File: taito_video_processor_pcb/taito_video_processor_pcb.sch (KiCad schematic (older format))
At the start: 237 parts, among them J1 14pin, J19 2pin, J2 14pin, J3 50pin, J6 50pin, Q1 2N3904, Q2 2N3904, Q3 2N3904, Q4 2N3904, Q5 2N3904, Q6 2N3904, Q7 2N3904, Q8 2N3905, SW1 SW_Push, U1 245_1, U10 4116, U100 LS00, U101 LS08, U102 LS10, U103 LS00, U104 157_1, U105 299_1, U106 299_1, U107 299_1, U108 299_1, U109 299_1, U11 4116, U110 299_1, U12 4116, U13 4116, U14 4116, U15 4116, U16 4116, U17 4116, U18 68A45, U19 86_2, U2 245_1, U20 86_1, U21 157_1, U22 LS32, U23 161_1, U24 LS04, U25 374_1, U26 4116, U27 4116, U28 4116, U29 4116, U3 2114, U30 4116, U31 4116, U32 4116, U33 4116, U34 LS374, U35 153_1, U36 LS74, U37 LS08, U38 74S113, U39 LS04, U4 2114, U40 7417, U41 4116, U42 4116, U43 4116, U44 4116, U45 4116, U46 4116, U47 4116, U48 4116, U49 LS32, U5 157_1, U50 86_3, U51 LS86, U52 153_1, U53 153_1, U54 153_1, U55 157_1, U56 2148_1, U57 2148_2, U58 7417, U59 4116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

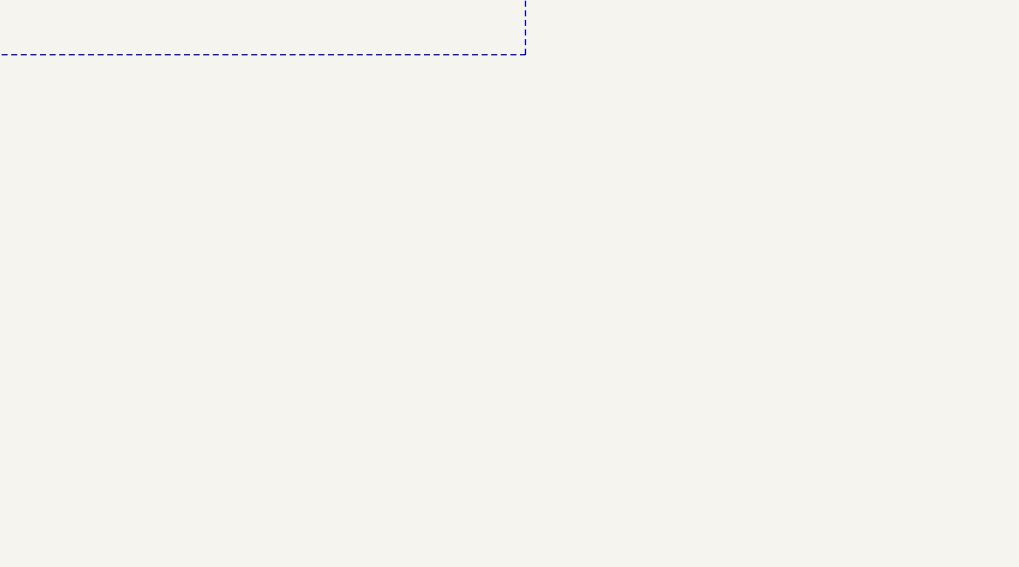
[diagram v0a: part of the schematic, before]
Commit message: Continued layout
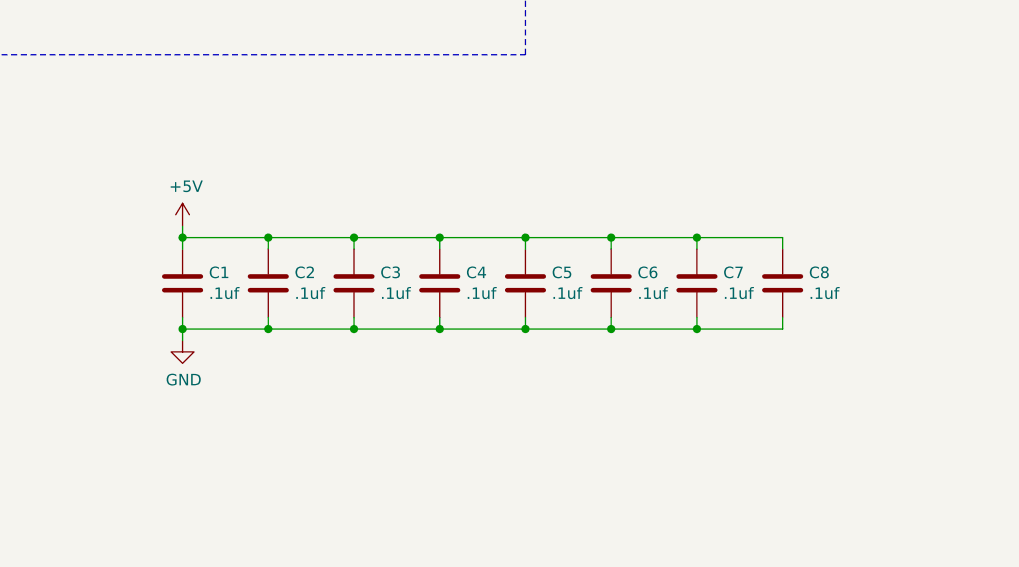
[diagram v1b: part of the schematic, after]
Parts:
- added C1, C2, C3, C4, C5, C6, C7, C8: .1uf, symbol Device:C
- J3, J6: footprint (none) -> taito_video_processor_pcb:50Pin
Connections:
- net +5V: now also C1.1, C2.1, C3.1, C4.1, C5.1, C6.1, C7.1, C8.1
- net GND: now also C1.2, C2.2, C3.2, C4.2, C5.2, C6.2, C7.2, C8.2
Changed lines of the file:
@@
 F 0 "J3" H 1400 3675 30  0000 L CNN
 F 1 "50pin" V 1425 3450 30  0000 L CNN
-F 2 "" H 1425 3425 30  0001 C CNN
+F 2 "taito_video_processor_pcb:50Pin" H 1425 3425 30  0001 C CNN
 F 3 "" H 1425 3425 30  0001 C CNN
 	1    1425 3425
@@
 F 0 "J6" H 31603 13430 30  0000 L CNN
 F 1 "50pin" H 31603 13370 30  0000 L CNN
-F 2 "" H 31525 13375 30  0001 C CNN
+F 2 "taito_video_processor_pcb:50Pin" H 31525 13375 30  0001 C CNN
 F 3 "" H 31525 13375 30  0001 C CNN
 	1    31525 13375
@@
 Wire Notes Line
 	28900 16275 28900 10600
+$Comp
+L Device:C C4
+U 1 1 61171227
+P 28525 17275
+F 0 "C4" H 28640 17321 50  0000 L CNN
+F 1 ".1uf" H 28640 17230 50  0000 L CNN
+F 2 "" H 28563 17125 50  0001 C CNN
+F 3 "~" H 28525 17275 50  0001 C CNN
+	1    28525 17275
+	1    0    0    -1
+$EndComp
+$Comp
+L Device:C C5
+U 1 1 61175975
+P 28900 17275
+F 0 "C5" H 29015 17321 50  0000 L CNN
+F 1 ".1uf" H 29015 17230 50  0000 L CNN
+F 2 "" H 28938 17125 50  0001 C CNN
+F 3 "~" H 28900 17275 50  0001 C CNN
+	1    28900 17275
+	1    0    0    -1
+$EndComp
+$Comp
+L Device:C C6
+U 1 1 61179FCE
+P 29275 17275
+F 0 "C6" H 29390 17321 50  0000 L CNN
+F 1 ".1uf" H 29390 17230 50  0000 L CNN
+F 2 "" H 29313 17125 50  0001 C CNN
+F 3 "~" H 29275 17275 50  0001 C CNN
+	1    29275 17275
+	1    0    0    -1
+$EndComp
+$Comp
+L Device:C C7
+U 1 1 6117E636
+P 29650 17275
+F 0 "C7" H 29765 17321 50  0000 L CNN
+F 1 ".1uf" H 29765 17230 50  0000 L CNN
+F 2 "" H 29688 17125 50  0001 C CNN
+F 3 "~" H 29650 17275 50  0001 C CNN
+	1    29650 17275
+	1    0    0    -1
+$EndComp
+$Comp
+L Device:C C8
+U 1 1 61182C28
+P 30025 17275
+F 0 "C8" H 30140 17321 50  0000 L CNN
+F 1 ".1uf" H 30140 17230 50  0000 L CNN
+F 2 "" H 30063 17125 50  0001 C CNN
+F 3 "~" H 30025 17275 50  0001 C CNN
+	1    30025 17275
+	1    0    0    -1
+$EndComp
+$Comp
+L Device:C C3
+U 1 1 6116CBF6
+P 28150 17275
+F 0 "C3" H 28265 17321 50  0000 L CNN
+F 1 ".1uf" H 28265 17230 50  0000 L CNN
+F 2 "" H 28188 17125 50  0001 C CNN
+F 3 "~" H 28150 17275 50  0001 C CNN
+	1    28150 17275
+	1    0    0    -1
+$EndComp
+$Comp
+L Device:C C2
+U 1 1 611685A7
+P 27775 17275
+F 0 "C2" H 27890 17321 50  0000 L CNN
+F 1 ".1uf" H 27890 17230 50  0000 L CNN
+F 2 "" H 27813 17125 50  0001 C CNN
+F 3 "~" H 27775 17275 50  0001 C CNN
+	1    27775 17275
+	1    0    0    -1
+$EndComp
+$Comp
+L Device:C C1
+U 1 1 61164136
+P 27400 17275
+F 0 "C1" H 27515 17321 50  0000 L CNN
+F 1 ".1uf" H 27515 17230 50  0000 L CNN
+F 2 "" H 27438 17125 50  0001 C CNN
+F 3 "~" H 27400 17275 50  0001 C CNN
+	1    27400 17275
+	1    0    0    -1
+$EndComp
+$Comp
+L power:+5V #PWR0350
+U 1 1 6152E23F
+P 27400 17025
+F 0 "#PWR0350" H 27400 16875 50  0001 C CNN
+F 1 "+5V" H 27415 17198 50  0000 C CNN
+F 2 "" H 27400 17025 50  0001 C CNN
+F 3 "" H 27400 17025 50  0001 C CNN
+	1    27400 17025
+	1    0    0    -1
+$EndComp
+Wire Wire Line
+	27400 17125 27400 17075
+Wire Wire Line
+	27400 17075 27775 17075
+Wire Wire Line
+	30025 17075 30025 17125
+Wire Wire Line
+	30025 17425 30025 17475
+Wire Wire Line
+	30025 17475 29650 17475
+Wire Wire Line
+	27400 17475 27400 17425
+Wire Wire Line
+	27775 17425 27775 17475
+Connection ~ 27775 17475
+Wire Wire Line
+	27775 17475 27400 17475
+Wire Wire Line
+	28150 17425 28150 17475
+Connection ~ 28150 17475
+Wire Wire Line
+	28150 17475 27775 17475
+Wire Wire Line
+	27775 17125 27775 17075
+Connection ~ 27775 17075
+Wire Wire Line
+	27775 17075 28150 17075
+Wire Wire Line
+	28150 17125 28150 17075
+Connection ~ 28150 17075
+Wire Wire Line
+	28150 17075 28525 17075
+Wire Wire Line
+	28525 17125 28525 17075
+Connection ~ 28525 17075
+Wire Wire Line
+	28525 17075 28900 17075
+Wire Wire Line
+	28900 17125 28900 17075
+Connection ~ 28900 17075
+Wire Wire Line
+	28900 17075 29275 17075
+Wire Wire Line
+	28525 17425 28525 17475
+Connection ~ 28525 17475
+Wire Wire Line
+	28525 17475 28150 17475
+Wire Wire Line
+	28900 17425 28900 17475
+Connection ~ 28900 17475
+Wire Wire Line
+	28900 17475 28525 17475
+Wire Wire Line
+	29650 17125 29650 17075
+Connection ~ 29650 17075
+Wire Wire Line
+	29650 17075 30025 17075
+Wire Wire Line
+	29275 17125 29275 17075
+Connection ~ 29275 17075
+Wire Wire Line
+	29275 17075 29650 17075
+Wire Wire Line
+	29275 17425 29275 17475
+Connection ~ 29275 17475
+Wire Wire Line
+	29275 17475 28900 17475
+Wire Wire Line
+	29650 17425 29650 17475
+Connection ~ 29650 17475
+Wire Wire Line
+	29650 17475 29275 17475
+Wire Wire Line
+	27400 17025 27400 17075
+Connection ~ 27400 17075
+$Comp
+L power:GND #PWR0351
+U 1 1 64BAC149
+P 27400 17525
+F 0 "#PWR0351" H 27400 17275 50  0001 C CNN
+F 1 "GND" H 27405 17352 50  0000 C CNN
+F 2 "" H 27400 17525 50  0001 C CNN
+F 3 "" H 27400 17525 50  0001 C CNN
+	1    27400 17525
+	1    0    0    -1
+$EndComp
+Wire Wire Line
+	27400 17525 27400 17475
+Connection ~ 27400 17475
 $EndSCHEMATC

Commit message: Placed components
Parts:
- added C10, C11, C12, C13, C15, C16, C17, C18, C19, C20, C21, C23, C24, C25, C26, C27, C28, C29, C30, C32, C33, C34, C35, C36, C37, C38, C39, C40, C41, C43, C46, C47, C48, C49, C50, C51, C52, C53, C54, C55, C56, C57, C58, C59, C60, C62, C64, C66, C67, C68, C69, C70, C71, C72, C73, C74, C75, C76, C78, C79, C81, C82, C87: .1uf, taito_video_processor_pcb:GenericComp, symbol Device:C
- added R11, R12, R22, R23, R24, R25, R26, R27, R9: ?, taito_video_processor_pcb:GenericComp, symbol Device:R_US
- C1, C14, C2, C3, C31, C4, C5, C6, C65, C7, C8, R1, R10, R13, R14, R15, R16, R17, R18, R19, R2, R20, R21, R28, R29, R3, R30, R31, R32, R33, R34, R35, R36, R39, R4, R40, R41, R42, R43, R44, R5, R6, R7, R8: footprint (none) -> taito_video_processor_pcb:GenericComp
- C22, C42, C44, C45, C61, C63, C77, C80, C9: footprint (none) -> taito_video_processor_pcb:CapA
- FB1, FB2, FB3, FB4, FB5, FB6, FB7: footprint (none) -> taito_video_processor_pcb:FB
- J1, J2: footprint (none) -> taito_video_processor_pcb:con_14pin
- J19: footprint (none) -> taito_video_processor_pcb:con_2pin
- Q1, Q2, Q3, Q4, Q5, Q6, Q7, Q8: footprint (none) -> taito_video_processor_pcb:Trans
- RP1, RP2, RP3, RP4, RP5: footprint (none) -> taito_video_processor_pcb:RP
- TP1, TP2, TP3, TP4: footprint (none) -> taito_video_processor_pcb:TPA
- Y1: footprint (none) -> taito_video_processor_pcb:Crystal
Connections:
- net +12V: now also C16.1, C18.1, C19.1, C21.1, C36.1, C37.1, C55.1, C59.1, C72.1, C76.1, C87.1
- net +5V: now also C10.1, C11.1, C12.1, C13.1, C15.1, C17.1, C20.1, C23.1, C26.1, C27.1, C28.1, C29.1, C30.1, C32.1, C35.1, C39.1, C41.1, C50.1, C51.1, C52.1, C56.1, C60.1, C64.1, C66.1, C67.1, C68.1, C69.1, C70.1, C71.1, C75.1, C79.1, C81.1, C82.1
- net -5V: now also C33.1, C34.1, C38.1, C40.1, C43.1, C53.1, C54.1, C57.1, C58.1, C62.1, C73.1, C74.1, C78.1
- net GND: now also C10.2, C11.2, C12.2, C13.2, C15.2, C16.2, C17.2, C18.2, C19.2, C20.2, C21.2, C23.2, C24.2, C25.2, C26.2, C27.2, C28.2, C29.2, C30.2, C32.2, C33.2, C34.2, C35.2, C36.2, C37.2, C38.2, C39.2, C40.2, C41.2, C43.2, C46.2, C47.2, C48.2, C49.2, C50.2, C51.2, C52.2, C53.2, C54.2, C55.2, C56.2, C57.2, C58.2, C59.2, C60.2, C62.2, C64.2, C66.2, C67.2, C68.2, C69.2, C70.2, C71.2, C72.2, C73.2, C74.2, C75.2, C76.2, C78.2, C79.2, C81.2, C82.2, C87.2
- net M0: now also R25.1; no longer U54.7
- net M1: now also R27.1; no longer U53.9
- net M2: now also R26.1; no longer U53.7
- net M3: now also R11.1; no longer U35.9
- net M4: now also R24.1; no longer U35.7
- net M5: now also R23.1; no longer U52.9
- net M6: now also R22.1; no longer U52.7
- net _BLUE_: now also C47.1
- net _CS_: now also C25.1
- net _GREEN_: now also C48.1
- net _HS_: now also C46.1
- net _RED_: now also C49.1
- net _VS_: now also C24.1
- net ~CAS: now also R9.2; no longer RP1.2
- net ~EVEN1: now also U67.5; no longer U67.2
- net ~ODD1: now also U67.2; no longer U67.5
- net ~RAS: now also R12.1; no longer U37.8
- net at Q1.1 (E), Q2.3 (C), Q3.3 (C)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: now also Q4.3 (C), Q5.3 (C), Q6.3 (C), Q7.3 (C), R31.1, R32.1, R33.1, R47.1
- net at U67.6: now also R36.2; no longer R21.2
- net at U67.3: now also R21.2; no longer R36.2
- net MUX: no longer names the net of U36.11 (2CLK), U38.9 (Q)
- new net: R22.2, U52.7
- new net: R23.2, U52.9
- new net: R24.2, U35.7
- new net: R11.2, U35.9
- new net: R26.2, U53.7
- new net: R27.2, U53.9
- new net: R25.2, U54.7
- new net: R12.2, U37.8
- new net ~CAS1: R9.1, RP1.2
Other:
- moved on the sheet: C1, C2, C3, C4, C5, C6, C7, C8, U35, U52, U53, U54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
